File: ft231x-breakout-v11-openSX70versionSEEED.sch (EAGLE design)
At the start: 24 parts, among them J1 XF2L-0625-1, Q1 2N7002, U1 FTS31XS-U

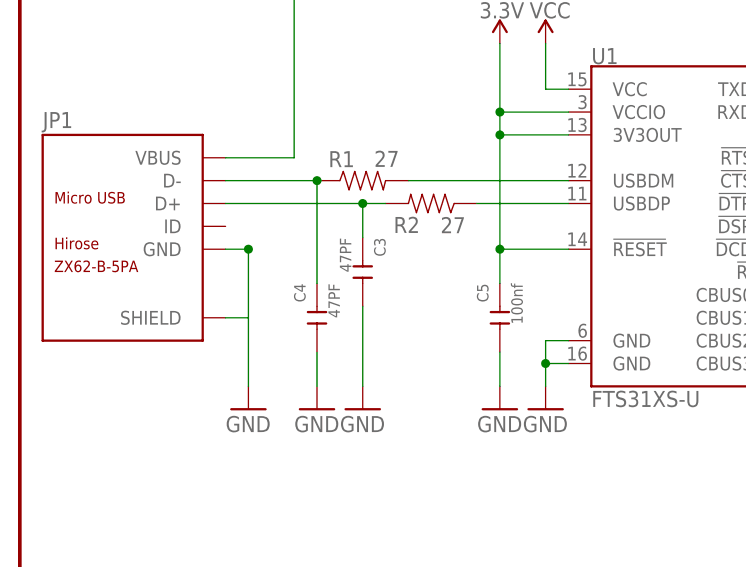
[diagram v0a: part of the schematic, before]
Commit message: New Breakout WIP
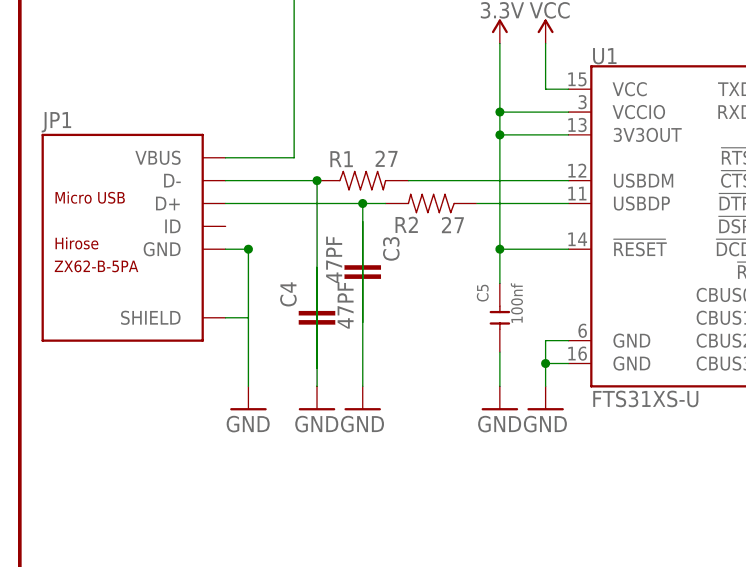
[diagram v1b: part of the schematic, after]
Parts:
- C3, C4: device Seeed-Capacitor-2016:CERAMIC-47PF-50V-5%-NP0(0402) -> Common-Parts-Library-Eagle:CC0603KRX7R9BB473
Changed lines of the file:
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@@
 <part name="U1" library="SparkFun-DigitalIC" deviceset="FT231X" device="S" value="FTS31XS-U"/>
 <part name="C2" library="Seeed-Capacitor" deviceset="CERAMIC-100NF-50V-10%-X7R(0603)" device="" value="100nf"/>
-<part name="C3" library="Seeed-Capacitor-2016" deviceset="CERAMIC-47PF-50V-5%-NP0(0402)" device="" value="47PF"/>
-<part name="C4" library="Seeed-Capacitor-2016" deviceset="CERAMIC-47PF-50V-5%-NP0(0402)" device="" value="47PF"/>
+<part name="C3" library="Common-Parts-Library-Eagle" deviceset="CC0603KRX7R9BB473" device="" value="47PF"/>
+<part name="C4" library="Common-Parts-Library-Eagle" deviceset="CC0603KRX7R9BB473" device="" value="47PF"/>
 <part name="R1" library="SparkFun-Resistors" deviceset="27OHM1/10W1%(0603)" device="0603-RES" value="27"/>
 <part name="R2" library="SparkFun-Resistors" deviceset="27OHM1/10W1%(0603)" device="0603-RES" value="27"/>
@@
 <pinref part="C3" gate="G$1" pin="1"/>
 <wire x1="40.64" y1="134.62" x2="38.1" y2="134.62" width="0.1524" layer="91"/>
-<wire x1="38.1" y1="134.62" x2="38.1" y2="130.81" width="0.1524" layer="91"/>
+<wire x1="38.1" y1="134.62" x2="38.1" y2="121.412" width="0.1524" layer="91"/>
 <wire x1="38.1" y1="134.62" x2="22.86" y2="134.62" width="0.1524" layer="91"/>
 <junction x="38.1" y="134.62"/>
@@
 <pinref part="R1" gate="G$1" pin="1"/>
 <pinref part="C4" gate="G$1" pin="1"/>
-<wire x1="33.02" y1="137.16" x2="33.02" y2="125.73" width="0.1524" layer="91"/>
+<wire x1="33.02" y1="137.16" x2="33.02" y2="116.332" width="0.1524" layer="91"/>
 <junction x="33.02" y="137.16"/>
 <pinref part="JP1" gate="G$1" pin="D-"/>
@@
 <pinref part="C4" gate="G$1" pin="2"/>
 <pinref part="GND1" gate="1" pin="GND"/>
-<wire x1="33.02" y1="114.3" x2="33.02" y2="118.11" width="0.1524" layer="91"/>
+<wire x1="33.02" y1="114.3" x2="33.02" y2="127.508" width="0.1524" layer="91"/>
 </segment>
 <segment>
 <pinref part="C3" gate="G$1" pin="2"/>
 <pinref part="GND2" gate="1" pin="GND"/>
-<wire x1="38.1" y1="114.3" x2="38.1" y2="123.19" width="0.1524" layer="91"/>
+<wire x1="38.1" y1="114.3" x2="38.1" y2="132.588" width="0.1524" layer="91"/>
 </segment>
 <segment>
